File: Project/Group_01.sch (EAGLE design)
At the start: 29 parts, among them J1 POWER_JACKPTH_LOCK, U1 +12v, U3 TCA9546APWR, U4 TMUX1208

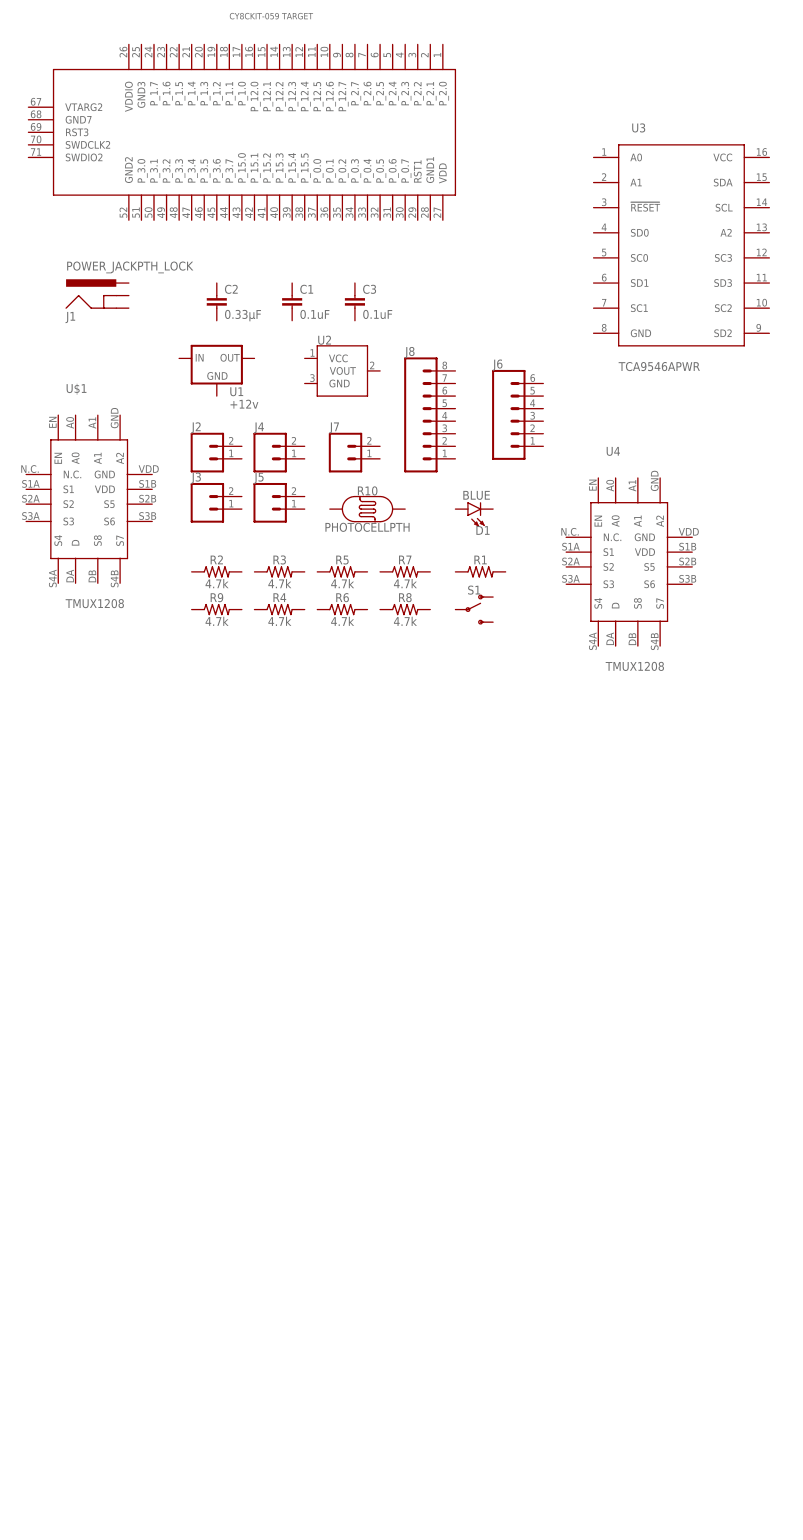
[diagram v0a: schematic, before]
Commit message: Schematics changes
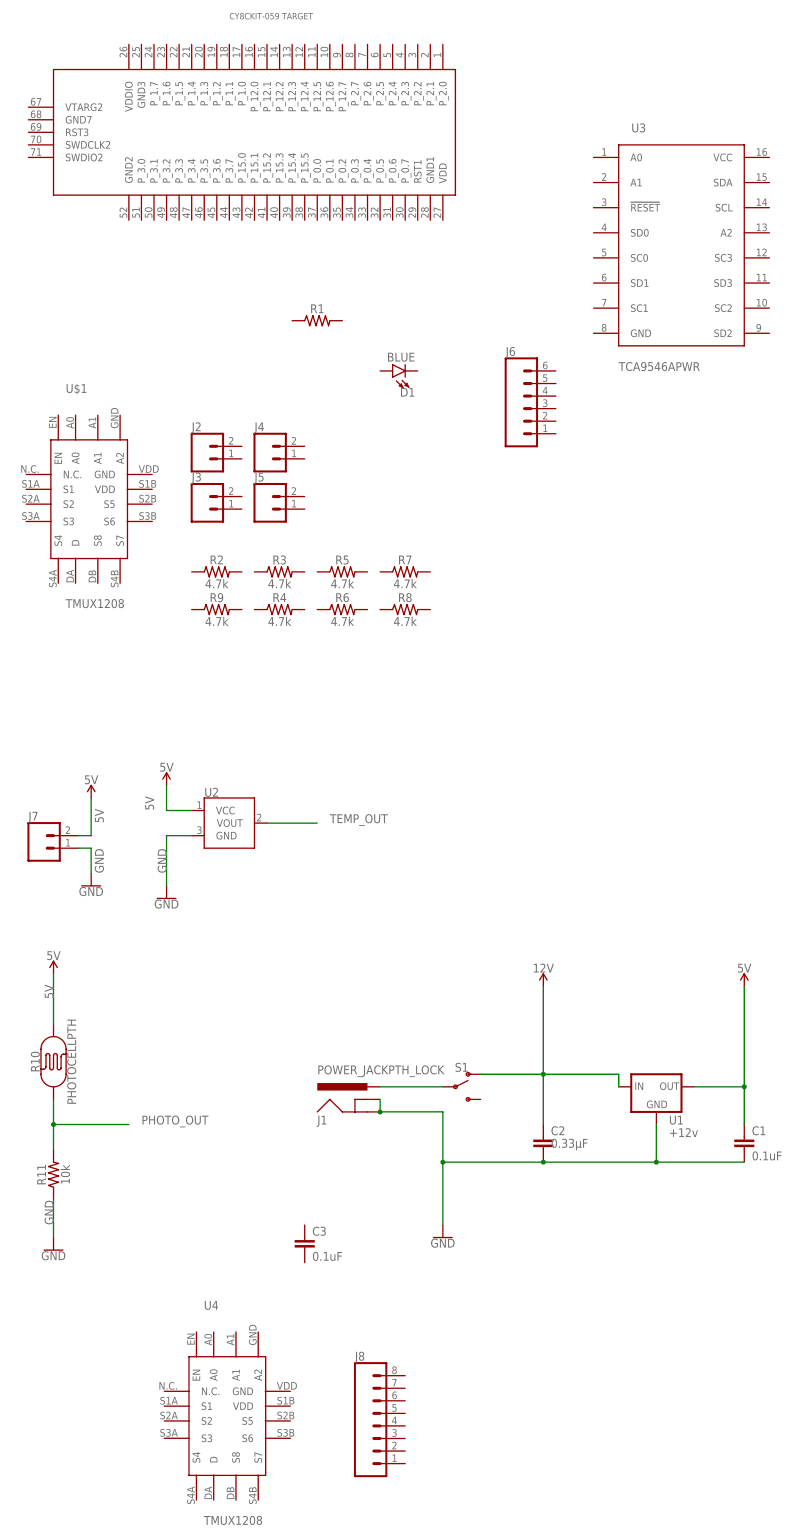
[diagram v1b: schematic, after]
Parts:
- added R11: 10k, SparkFun-Resistors:10KOHM-0603-1/10W-1%
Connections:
- new net 12V: C2.1, S1.O, U1.IN
- new net 5V: C1.1, J7.2, R10.P$2, U1.OUT, U2.VCC
- new net GND: C1.2, C2.2, J1.GND, J1.GNDBREAK, J7.1, R11.1, U1.GND, U2.GND
- new net N$1: J1.PWR, S1.P
- new net PHOTO_OUT: R10.P$1, R11.2
- new net TEMP_OUT: U2.VOUT
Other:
- moved on the sheet: C1, C2, C3, D1, J1, J6, J7, J8, R1, R10, S1, U1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
